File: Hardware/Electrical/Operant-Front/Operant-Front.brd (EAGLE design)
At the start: 160 x 100 mm, 13 parts

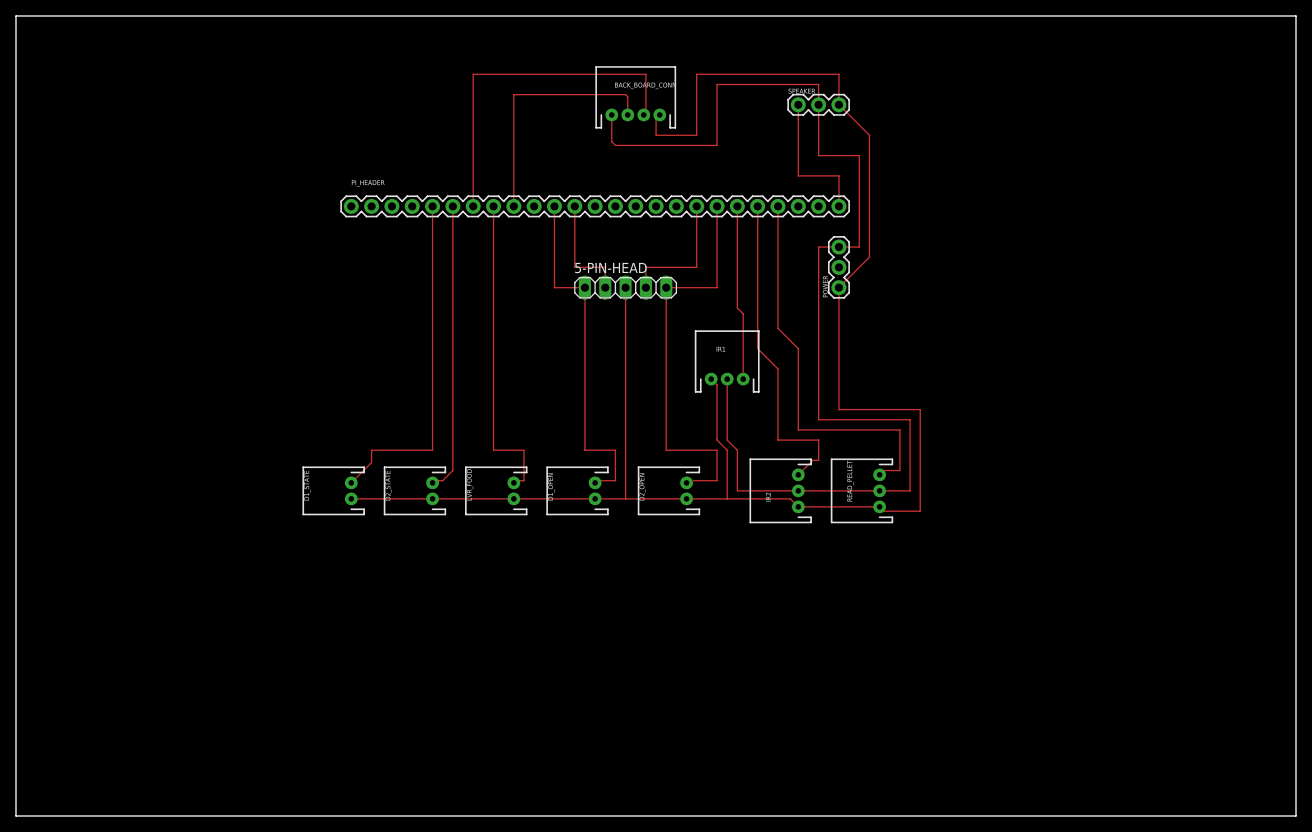
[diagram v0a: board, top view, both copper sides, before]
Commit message: Final version for standard operant board
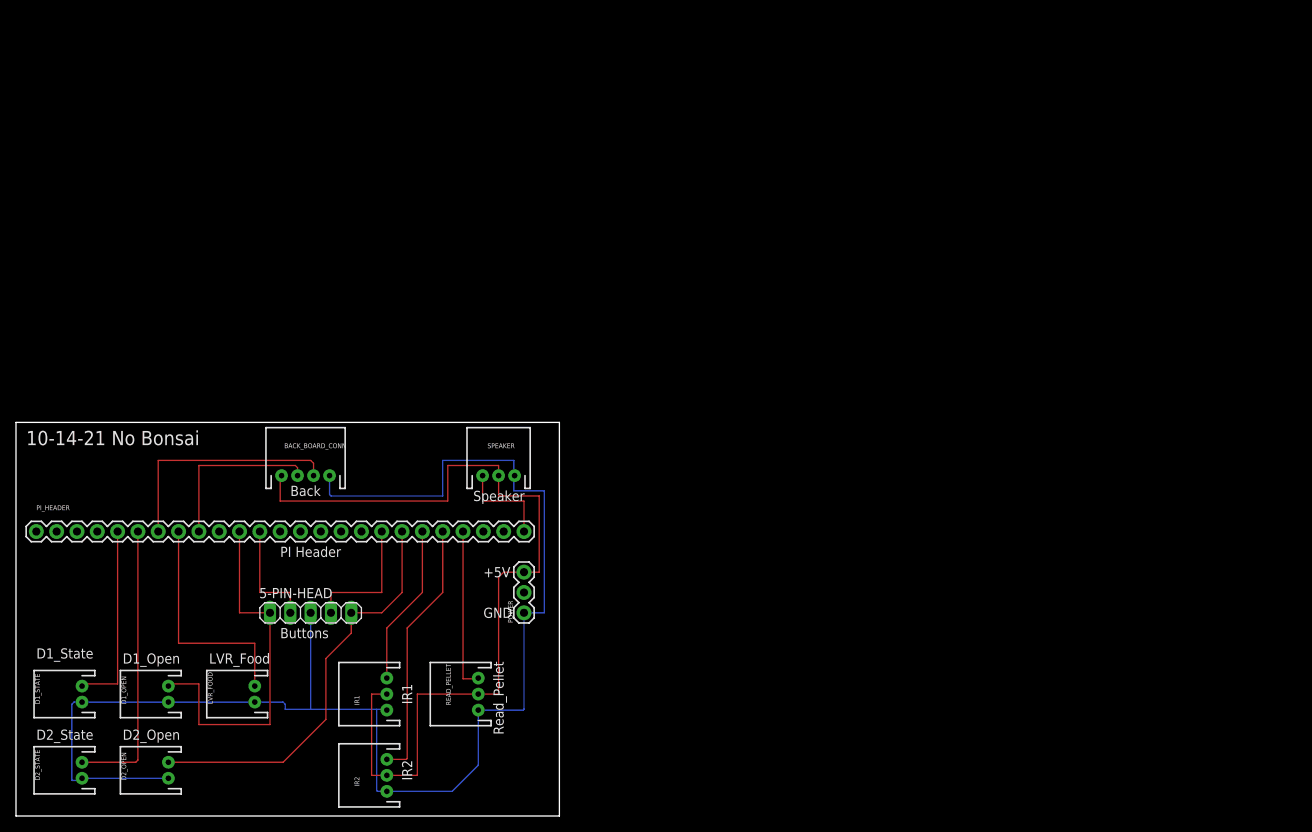
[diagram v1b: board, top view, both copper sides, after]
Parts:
- POWER: value 455-1750-1-ND -> (none)
- SPEAKER: value 455-1750-1-ND -> (none); device SparkFun-Connectors:1X03 -> SparkFun-Connectors:JST-3-PTH
- moved D2_OPEN 73.6 mm to (19.1, 5.71)
- moved IR2 62.5 mm to (46.4, 5.08)
- moved BACK_BOARD_CONN 61.1 mm to (36.2, 42.5)
- moved SPEAKER 59.6 mm to (60.3, 42.5)
- moved D1_OPEN 59.1 mm to (19.1, 15.2)
- moved IR1 58.0 mm to (46.4, 15.2), turned to 90 degrees
- moved 5-PIN-HEAD 56.6 mm to (36.8, 25.4)
- moved POWER 56.6 mm to (63.5, 25.4)
- moved PI_HEADER 56.6 mm to (2.54, 35.6)
- moved READ_PELLET 56.2 mm to (57.8, 15.2)
- moved D2_STATE 56.0 mm to (8.26, 5.71)
- moved D1_STATE 42.2 mm to (8.26, 15.2)
- moved LVR_FOOD 41.2 mm to (29.8, 15.2)
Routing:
- net GND: track 215.1 -> 178.4 mm
- net +5V: track 146.4 -> 111.5 mm
- net GPIO16: track 49.5 -> 20.4 mm
- net GPIO4: track 43.2 -> 23.6 mm
- net GPIO18: track 43.3 -> 30.0 mm
- net GPIO27: track 39.5 -> 28.8 mm
- net GPIO13: track 41.9 -> 32.8 mm
- net GPIO22: track 30.6 -> 21.7 mm
- net GPIO21: track 17.8 -> 12.2 mm
- net GPIO12: track 21.9 -> 20.2 mm
- net GPIO6: track 50.0 -> 51.6 mm
- net GPIO24: track 44.6 -> 45.8 mm
- net GPIO17: track 36.2 -> 35.7 mm
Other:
- board size 160 x 100 mm -> 67.9 x 49.2 mm
- board text added: "+5V"
- board text added: "10-14-21 No Bonsai"
- board text added: "Back"
- board text added: "Buttons"
- board text added: "D1_Open"
- board text added: "D1_State"
- board text added: "D2_Open"
- board text added: "D2_State"
- board text added: "GND"
- board text added: "IR1"
- board text added: "IR2"
- board text added: "LVR_Food"
- board text added: "PI Header"
- board text added: "Read_Pellet"
- board text added: "Speaker"
